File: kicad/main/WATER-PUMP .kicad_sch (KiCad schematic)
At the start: 10 parts, among them Q7 IRLML6344TRPBF, Q8 AO3401

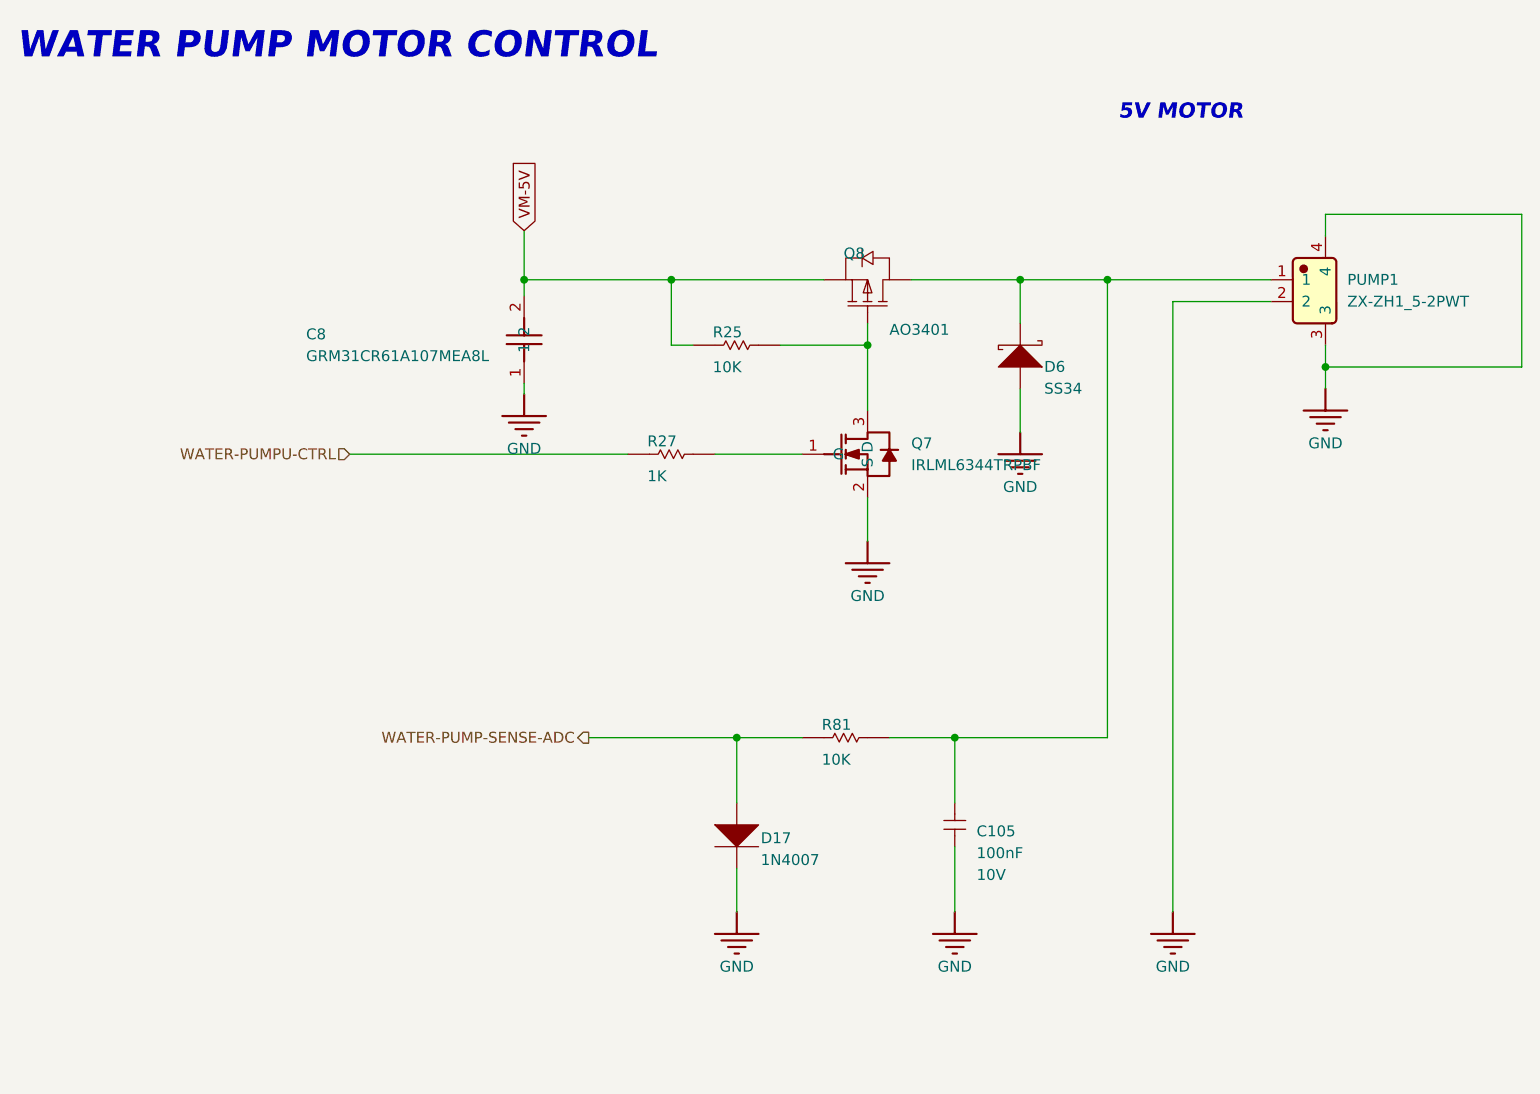
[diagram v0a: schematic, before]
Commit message: Schematic fixes, 1st round of review
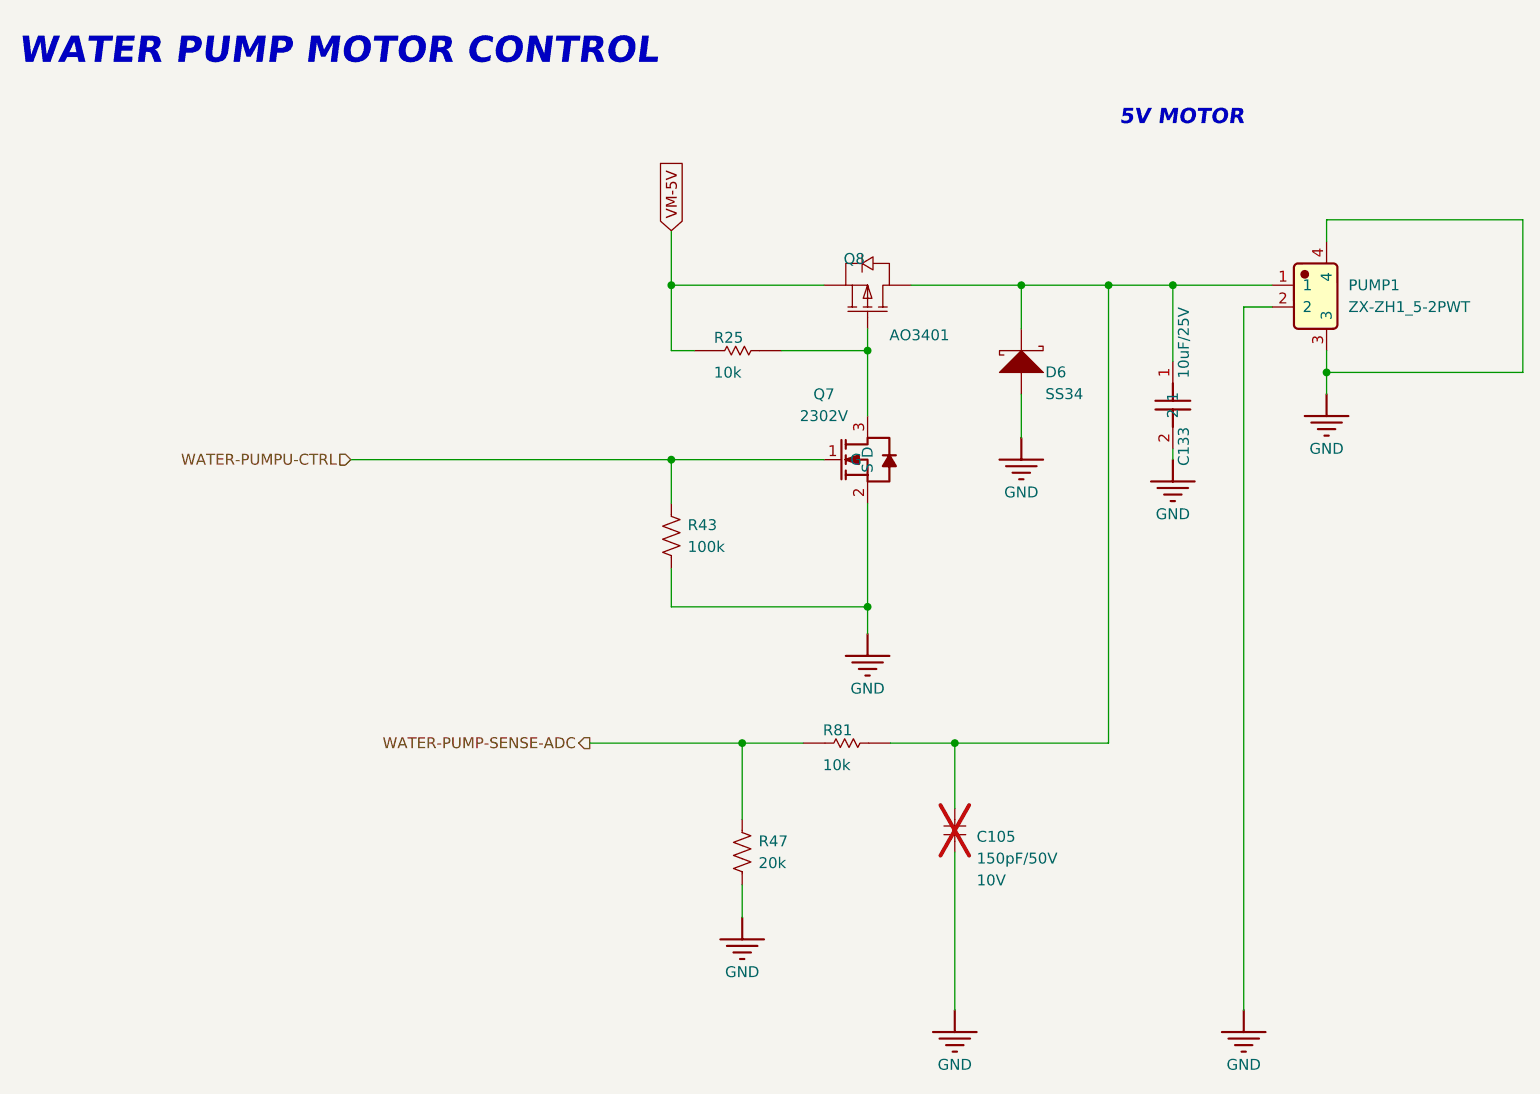
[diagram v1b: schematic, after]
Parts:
- removed C8: GRM31CR61A107MEA8L, JLCImport:GRM31CR61A107MEA8L, symbol JLCImport:GRM31CR61A107MEA8L
- removed D17: 1N4007, oomwoo_altium:SOD123, symbol DesignLibrary:WATER-PUMP_3_DIODE-1_DesignLibrary.SchLib
- removed Q7: IRLML6344TRPBF, JLCImport:IRLML6344TRPBF, symbol JLCImport:IRLML6344TRPBF
- removed R27: 1K, Resistor_SMD:R_0603_1608Metric, symbol DesignLibrary:WATER-PUMP_2_Resistor-1_DesignLibrary.SchLib
- added C133: 10uF/25V, Capacitor_SMD:C_0603_1608Metric, symbol JLCImport:CL21A106KBYQNNE
- added Q7: 2302V, JLCImport:2302V, symbol JLCImport:2302V
- added R43: 100k, Resistor_SMD:R_0603_1608Metric, symbol Device:R_US
- added R47: 20k, Resistor_SMD:R_0603_1608Metric, symbol Device:R_US
- C105: value 100nF -> 150pF/50V; MANUFACTURER * -> (none); Manufacturer (none) -> *; now not fitted
- D6: footprint oomwoo_altium:SMA -> Diode_SMD:D_SMA; LCSC (none) -> C22448055; MANUFACTURER * -> (none); Manufacturer (none) -> *
- Q8: LCSC (none) -> C15127; MANUFACTURER * -> (none); Manufacturer (none) -> *
- R25, R81: value 10K -> 10k; MANUFACTURER * -> (none); Manufacturer (none) -> *
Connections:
- net GND: now also C133.2, Q7.2 (S), R43.2, R47.2
- net WATER-PUMP-SENSE-ADC: now also R47.1
- net WATER-PUMPU-CTRL: now also Q7.1 (G), R43.1
- net at Q8.1 (G), R25.1: now also Q7.3 (D)
- net at C105.2, D6.2 (K), PUMP1.1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: now also C133.1
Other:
- moved on the sheet: D6, PUMP1, Q8, R25, R81
